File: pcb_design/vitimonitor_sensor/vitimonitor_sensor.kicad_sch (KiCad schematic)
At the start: 0 parts

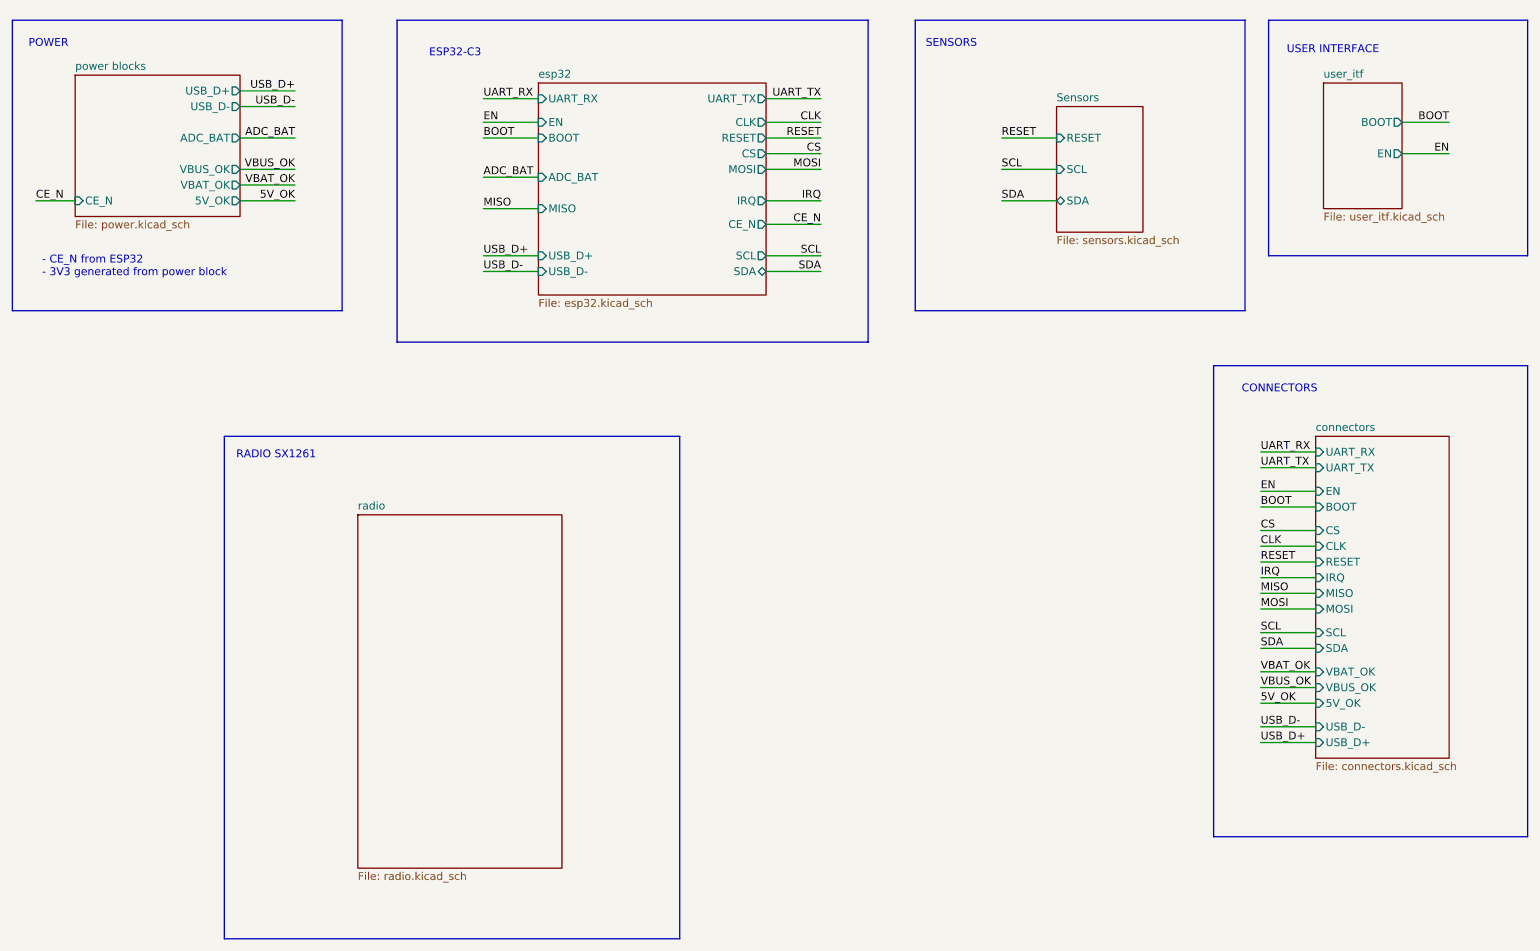
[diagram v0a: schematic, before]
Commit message: Changes due to a first review
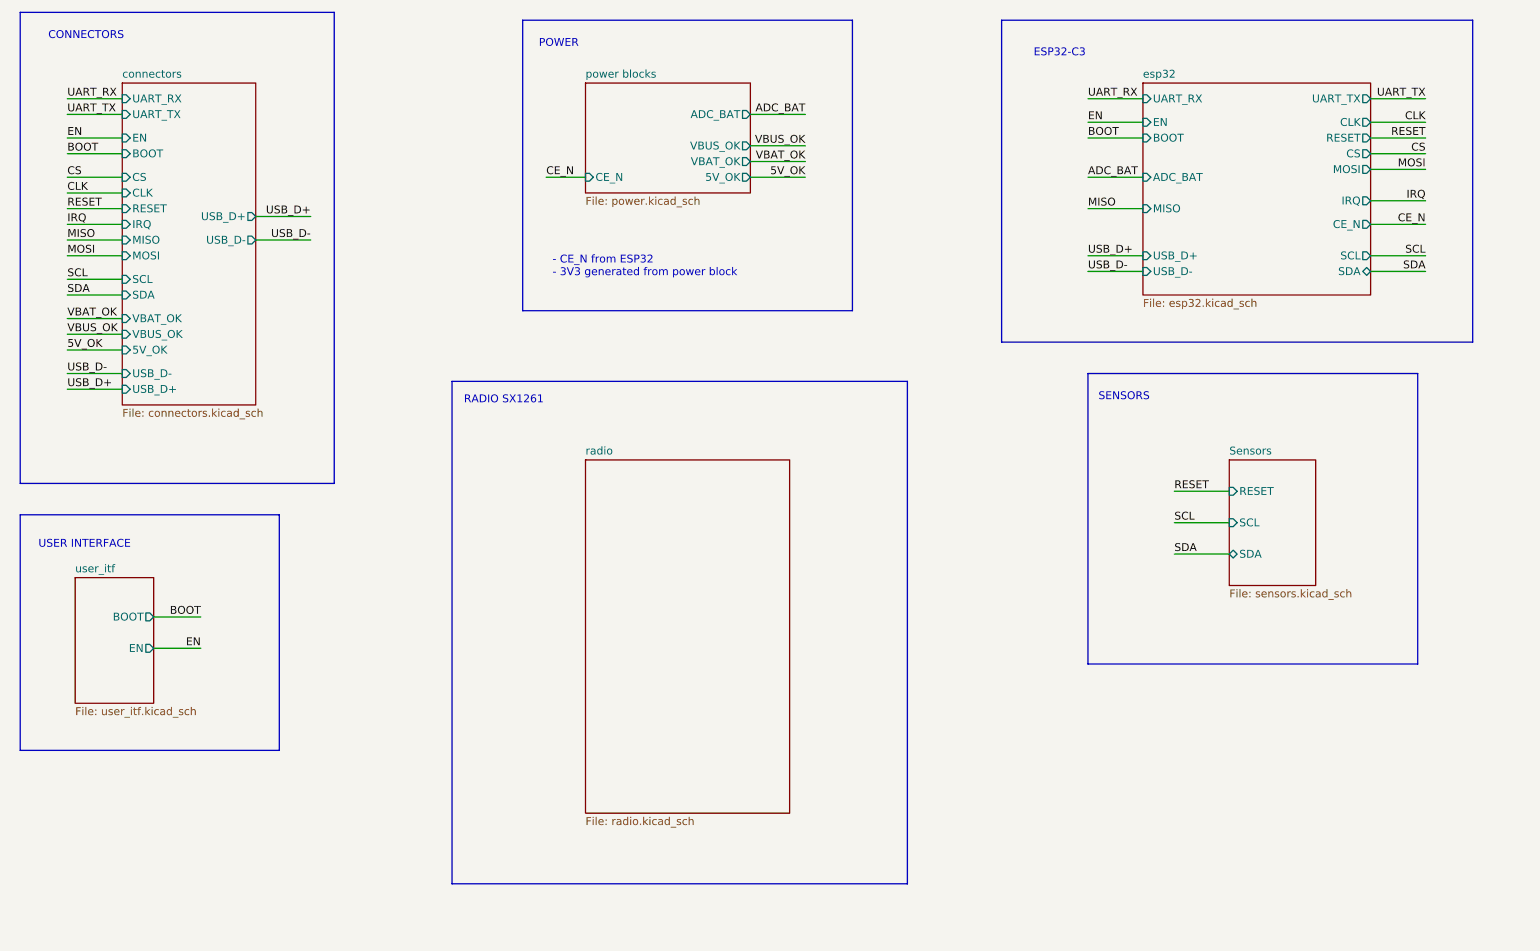
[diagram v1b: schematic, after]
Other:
- sheet power blocks ports: added none; removed USB_D+, USB_D-
